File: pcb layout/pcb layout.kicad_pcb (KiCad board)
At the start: 2 copper layers, 7 parts, among them U1 ESP32-DevKitC, U2 DHT11

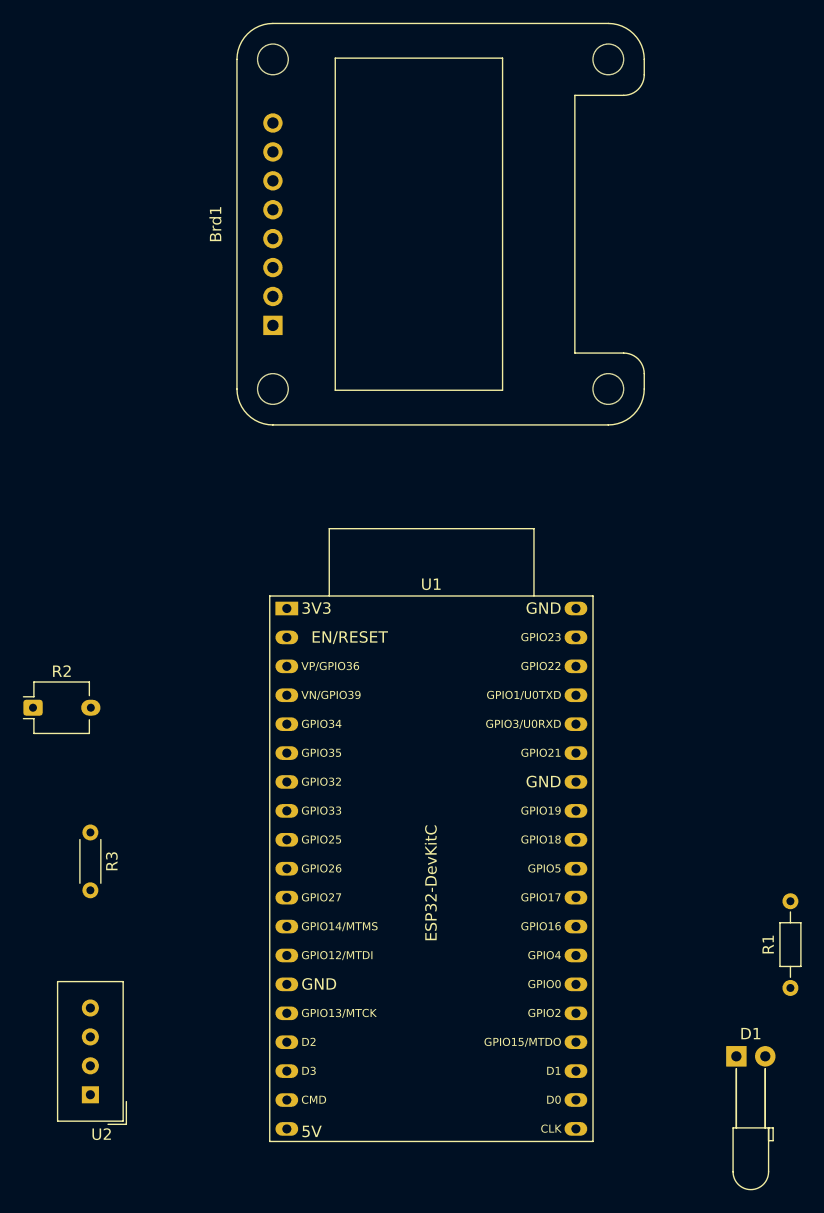
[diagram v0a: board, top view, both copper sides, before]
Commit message: feat: update pcb
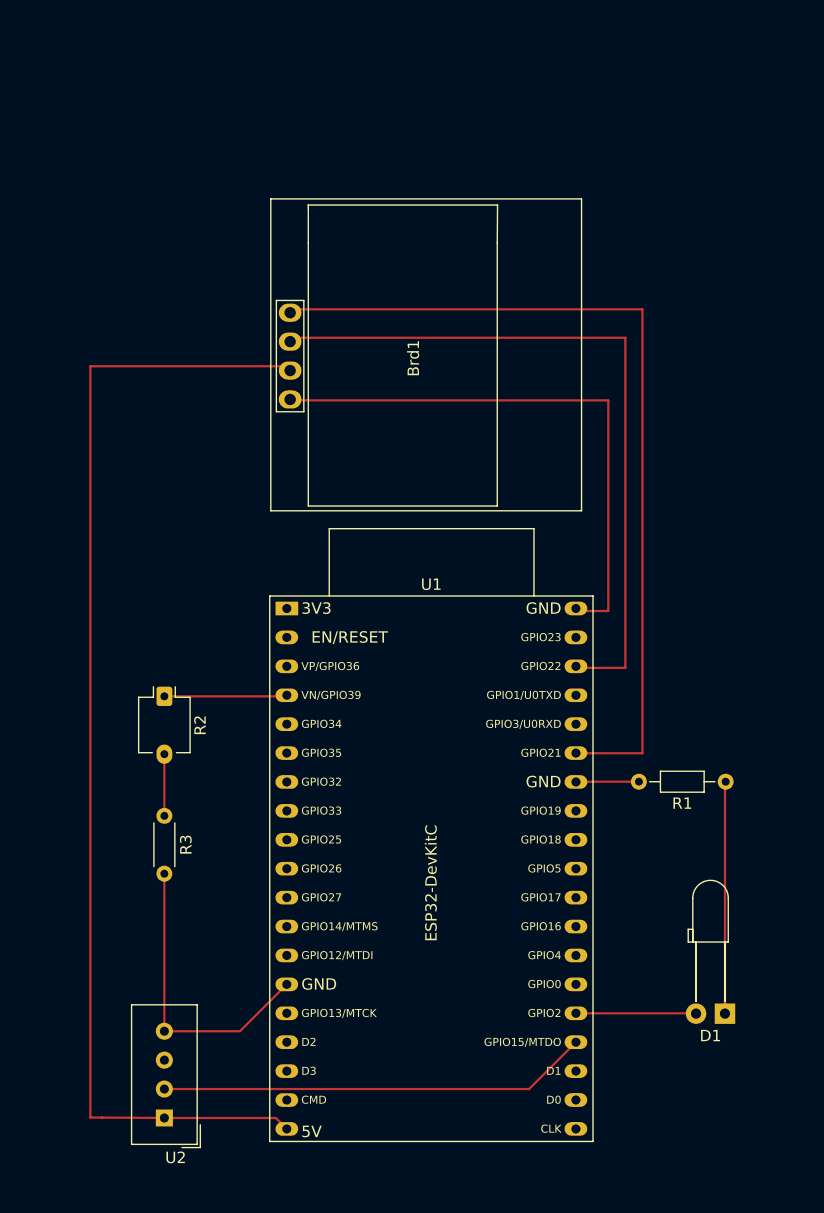
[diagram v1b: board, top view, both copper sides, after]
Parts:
- Brd1: footprint Display:Adafruit_SSD1306 -> SSD1306:128x64OLED
- moved R1 19.0 mm to (176.8, 121.0), turned to 180 degrees
- moved Brd1 12.5 mm to (149.2, 83.8)
- moved R2 11.6 mm to (127.5, 113.5), turned to -90 degrees
- moved U2 6.81 mm to (127.5, 150.5)
- moved R3 6.66 mm to (127.5, 124.0)
- moved D1 3.88 mm to (176.8, 141.4), turned to 180 degrees
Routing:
- net Net-(U1-MTDO/GPIO15/ADC2_CH3): track 0.00 -> 37.9 mm
- net Earth: track 0.00 -> 31.8 mm
- net Net-(D1-K): track 0.00 -> 20.4 mm
- net Net-(Brd1-VCC): track 0.00 -> 11.2 mm
- net Net-(U1-SENSOR_VN/GPIO39/ADC1_CH3): track 0.00 -> 10.8 mm
- net Net-(D1-A): track 0.00 -> 10.6 mm
- net Net-(R2-Pad2): track 0.00 -> 5.42 mm
